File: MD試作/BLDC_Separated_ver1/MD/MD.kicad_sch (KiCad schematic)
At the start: 1 part, among them J4 Conn_02x13_Odd_Even

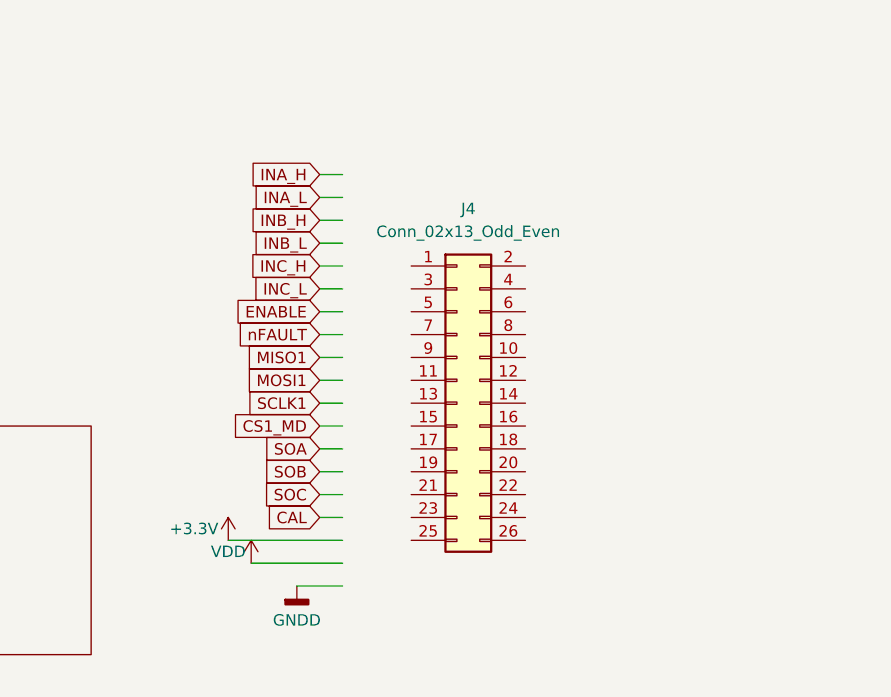
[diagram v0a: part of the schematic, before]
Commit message: かんせい
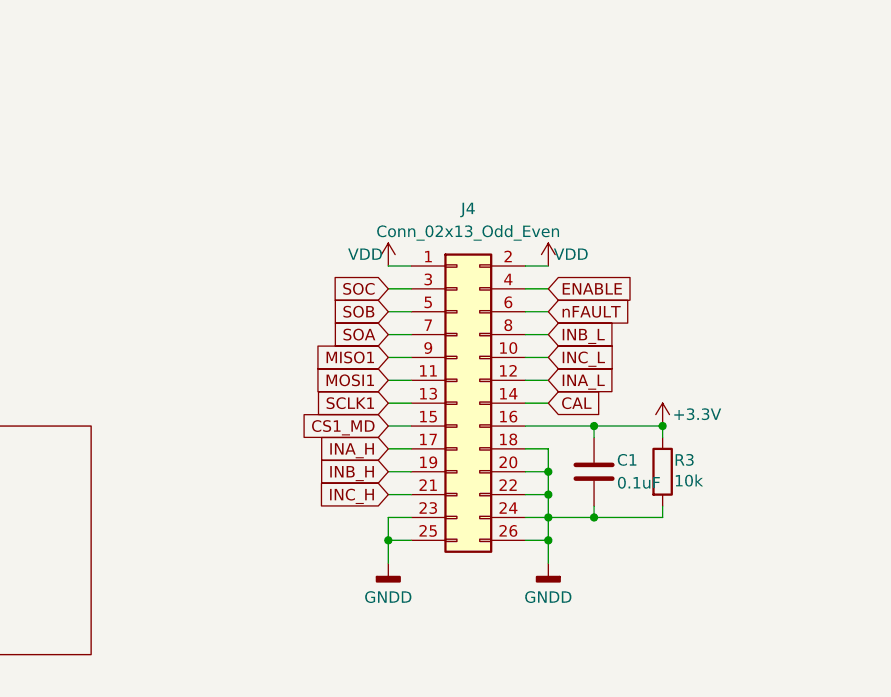
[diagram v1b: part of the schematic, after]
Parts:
- added C1: 0.1uF, Capacitor_SMD:C_0402_1005Metric, symbol Device:C
- added R3: 10k, Resistor_SMD:R_0402_1005Metric, symbol Device:R
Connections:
- net +3.3V: now also J4.16 (Pin_16), C1.1, R3.1
- net CAL: now also J4.14 (Pin_14)
- net CS1_MD: now also J4.15 (Pin_15)
- net ENABLE: now also J4.4 (Pin_4)
- net GNDD: now also J4.18 (Pin_18), J4.20 (Pin_20), J4.22 (Pin_22), J4.23 (Pin_23), J4.24 (Pin_24), J4.25 (Pin_25), J4.26 (Pin_26), C1.2, R3.2
- net INA_H: now also J4.17 (Pin_17)
- net INA_L: now also J4.12 (Pin_12)
- net INB_H: now also J4.19 (Pin_19)
- net INB_L: now also J4.8 (Pin_8)
- net INC_H: now also J4.21 (Pin_21)
- net INC_L: now also J4.10 (Pin_10)
- net MISO1: now also J4.9 (Pin_9)
- net MOSI1: now also J4.11 (Pin_11)
- net SCLK1: now also J4.13 (Pin_13)
- net SOA: now also J4.7 (Pin_7)
- net SOB: now also J4.5 (Pin_5)
- net SOC: now also J4.3 (Pin_3)
- net VDD: now also J4.1 (Pin_1), J4.2 (Pin_2)
- net nFAULT: now also J4.6 (Pin_6)
